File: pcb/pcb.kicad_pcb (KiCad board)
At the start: 4 copper layers, 48.3 x 68.5 mm, 52 parts, among them J1 Conn_02x09_Odd_Even, J10 Conn_01x04, J11 Conn_01x02, J12 Conn_01x02, J2 Conn_02x09_Odd_Even, J3 Conn_02x09_Odd_Even, J4 Conn_02x09_Odd_Even, J5 Jack-DC, J6 Conn_01x04, J7 Conn_01x05, J8 Conn_01x01, J9 Conn_01x02, U1 MCP23017, U2 MCP23017, U3 MCP23017, U4 MCP23017, U5 LMZ12002, U6 LMZ12002, U7 TXS0102, U8 TXS0102, X1 PLTWS7, Y1 Mount, Y2 Mount, Y3 Mount, Y4 Mount

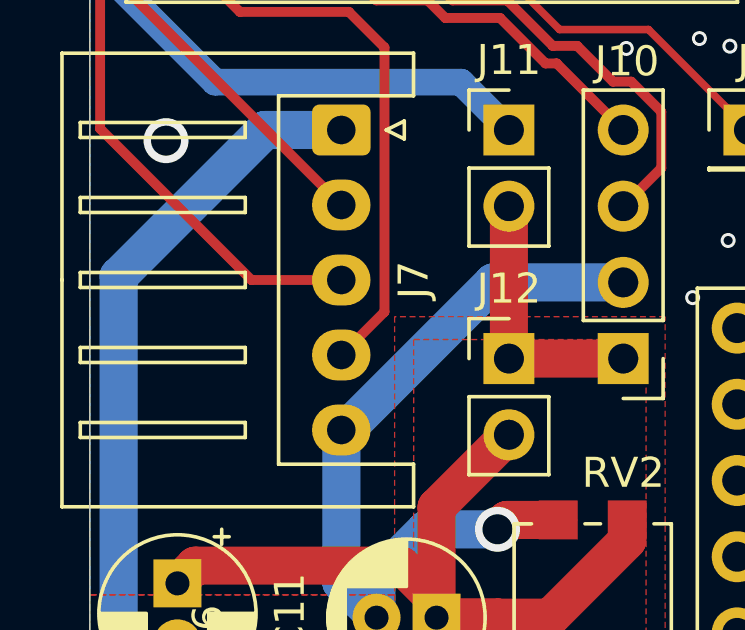
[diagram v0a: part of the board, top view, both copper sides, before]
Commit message: pull down
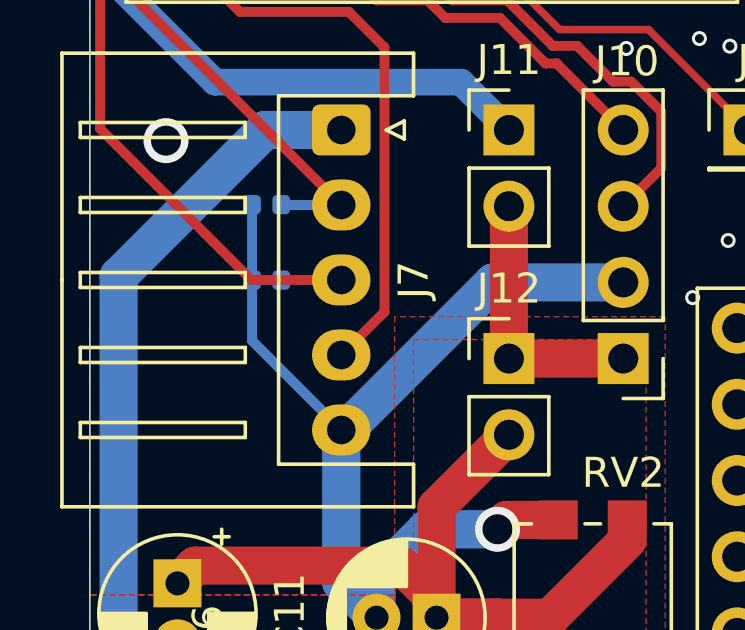
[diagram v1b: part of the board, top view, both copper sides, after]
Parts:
- added R7: 33k, Resistor_SMD:R_0402_1005Metric, B.Cu at (107.5, 103.6)
- added R8: 33k, Resistor_SMD:R_0402_1005Metric, B.Cu at (107.5, 101.0)
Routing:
- net GND: track 451.3 -> 460.0 mm
- net /dtr_3v3: track 31.7 -> 33.7 mm
- net /p2f_3v3: track 34.2 -> 36.2 mm

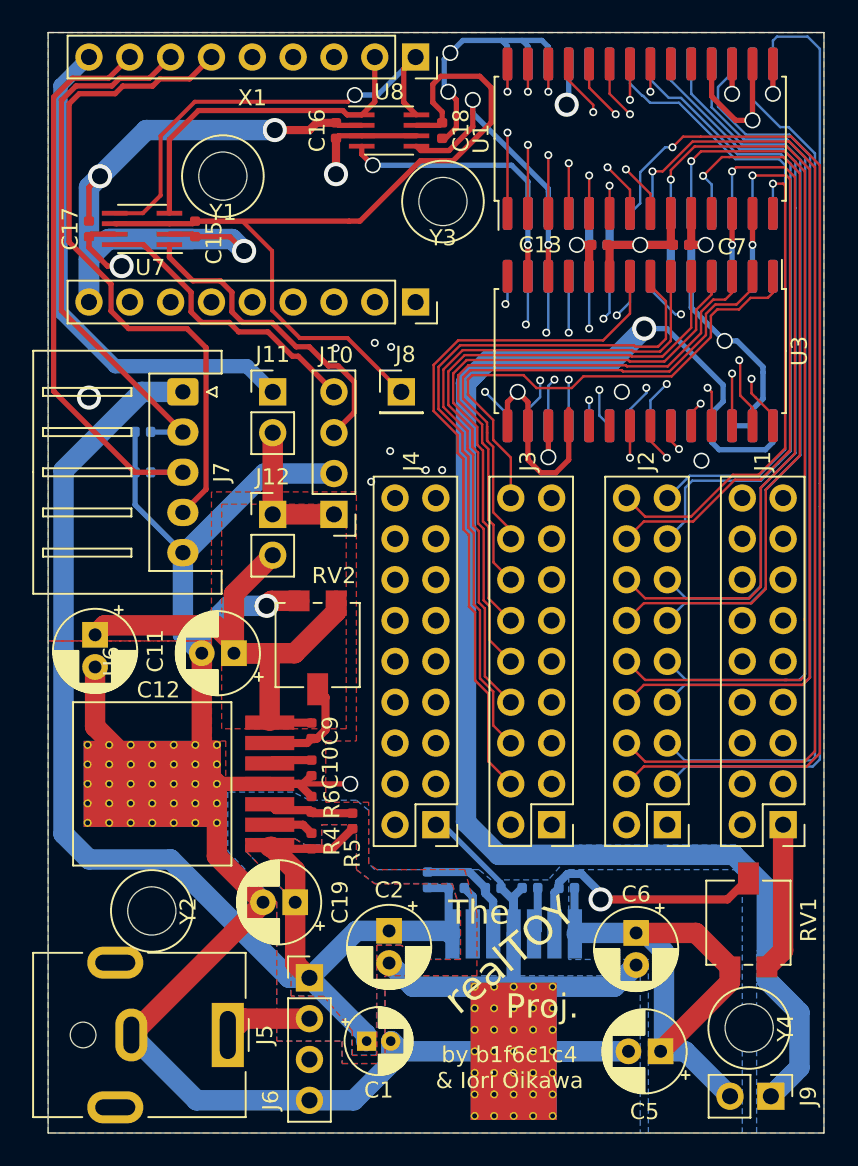
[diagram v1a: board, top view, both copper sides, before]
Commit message: pcb adjust
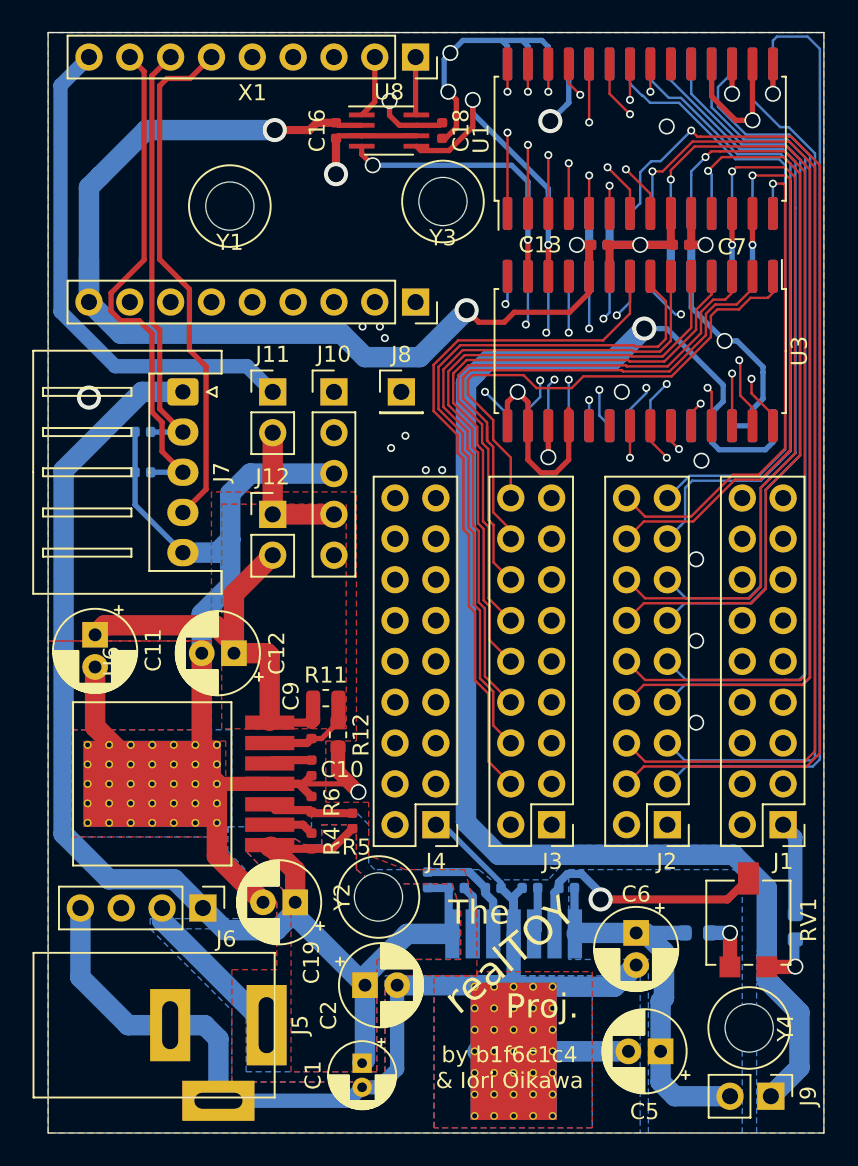
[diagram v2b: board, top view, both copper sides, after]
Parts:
- removed C15, C17: 100n, Capacitor_SMD:C_0402_1005Metric
- removed RV2: R_POT, Potentiometer_SMD:Potentiometer_Vishay_TS53YL_Vertical
- removed U7: TXS0102, kicad-lib:TI-R-PDSO-G8
- added R10: 1.02k, 0.5%, Resistor_SMD:R_0603_1608Metric, B.Cu at (148.1, 131.8)
- added R11: 5.36k, 0.5%, Resistor_SMD:R_0603_1608Metric, F.Cu at (118.9, 117.6)
- added R12: 1.02k, 0.5%, Resistor_SMD:R_0603_1608Metric, F.Cu at (119.6, 119.9)
- added R9: 2.15k, 0.5%, Resistor_SMD:R_0603_1608Metric, B.Cu at (142.0, 132.2)
- J10: value Conn_01x04 -> Conn_01x05; footprint Connector_PinHeader_2.54mm:PinHeader_1x04_P2.54mm_Vertical -> Connector_PinHeader_2.54mm:PinHeader_1x05_P2.54mm_Vertical
- J5: footprint Connector_BarrelJack:BarrelJack_CUI_PJ-063AH_Horizontal -> b1:KLDX-0202
- RV1: value R_POT -> 1k
- moved Y2 14.1 mm to (122.1, 130.0), turned to 270 degrees
- moved J6 7.93 mm to (111.2, 130.7), turned to 270 degrees
- moved J10 7.62 mm to (119.4, 98.6), turned to 0 degrees
- moved C2 3.70 mm to (121.3, 135.5), turned to 0 degrees
- moved Y1 1.91 mm to (112.9, 87.0)
- moved C1 1.40 mm to (121.1, 140.3), turned to 270 degrees
- moved J5 0.84 mm to (112.2, 137.9), turned to 90 degrees
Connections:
- J10 pad 1: /+5V -> /scl_3v3
- J10 pad 2: GND -> /sda_3v3
- J10 pad 3: /sda_5v -> GND
- J10 pad 4: /scl_5v -> /+5V
- RV1 pad 1: GND -> Net-(R10-Pad1)
- RV1 pad 3: /VADJ1 -> Net-(R9-Pad2)
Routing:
- net /+5V: track 37.7 -> 8.89 mm, vias 1 -> 0
- net /sda_5v: track 19.9 -> 0.00 mm
- net /scl_5v: track 18.1 -> 0.00 mm
- net /+3V3: track 56.5 -> 43.0 mm, vias 0 -> 1
- net /VADJ1: track 34.3 -> 24.7 mm
- net /f2p_3v3: track 41.7 -> 32.3 mm
- net /sda_3v3: track 21.3 -> 30.2 mm
- net /dtr_3v3: track 33.7 -> 26.6 mm
- net GND: track 460.0 -> 453.6 mm, vias 16 -> 18
- net /VADJ2: track 34.1 -> 29.1 mm
- net /p2f_3v3: track 36.2 -> 31.6 mm
- net /VIN0: track 5.50 -> 9.98 mm
- net Net-(R10-Pad1): track 0.00 -> 3.47 mm, vias 0 -> 1
- net Net-(R9-Pad2): track 0.00 -> 3.36 mm, vias 0 -> 1
- net /VIN: track 85.8 -> 83.0 mm
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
